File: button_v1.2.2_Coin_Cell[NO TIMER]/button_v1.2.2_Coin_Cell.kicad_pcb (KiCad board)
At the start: 2 copper layers, 21 x 47.8 mm, 18 parts, among them J1 Conn_01x05_Female, SW1 SW_Push, SW2 SW_Push, U1 TPS61097A, X1 ESP-12E

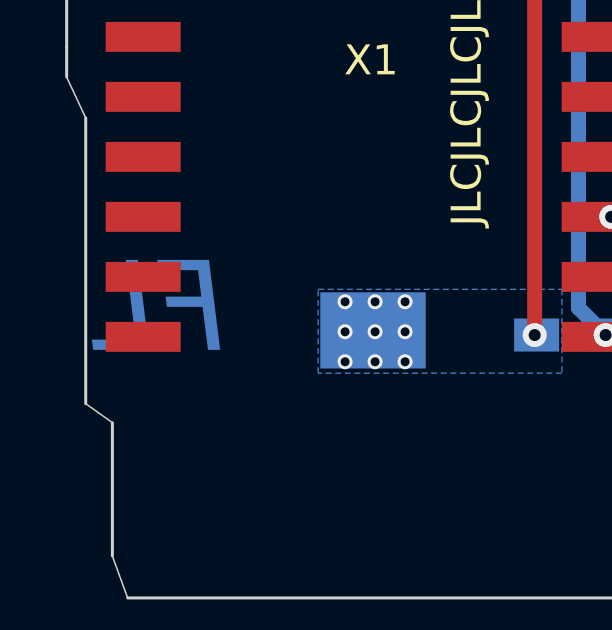
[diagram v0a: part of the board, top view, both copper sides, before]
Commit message: 23.02 00:38
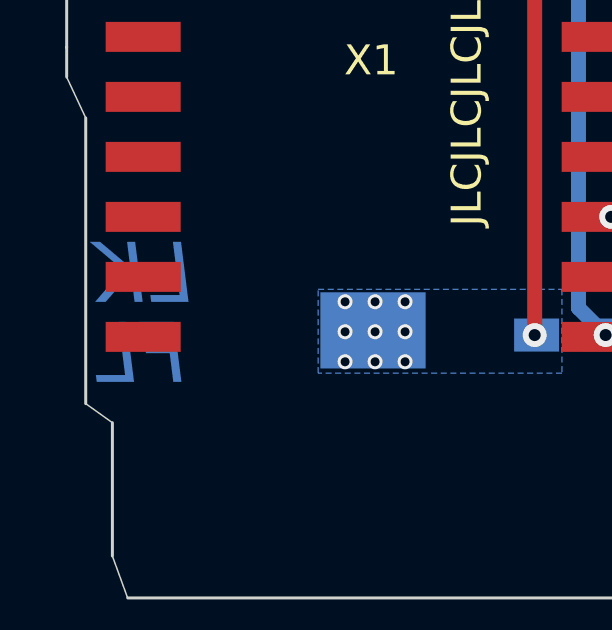
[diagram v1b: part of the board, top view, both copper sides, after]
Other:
- board text added: "LK"
